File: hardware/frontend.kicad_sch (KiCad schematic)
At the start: 33 parts, among them J10 Conn_01x03_MountingPin, J11 Conn_01x11_MountingPin, J7 EXT_NTC, J8 EXT_NTC, J9 Conn_01x03_MountingPin, Q4 IPTC025N15NM6, Q5 IPTC025N15NM6, Q6 BSS127S, U5 BQ769x2

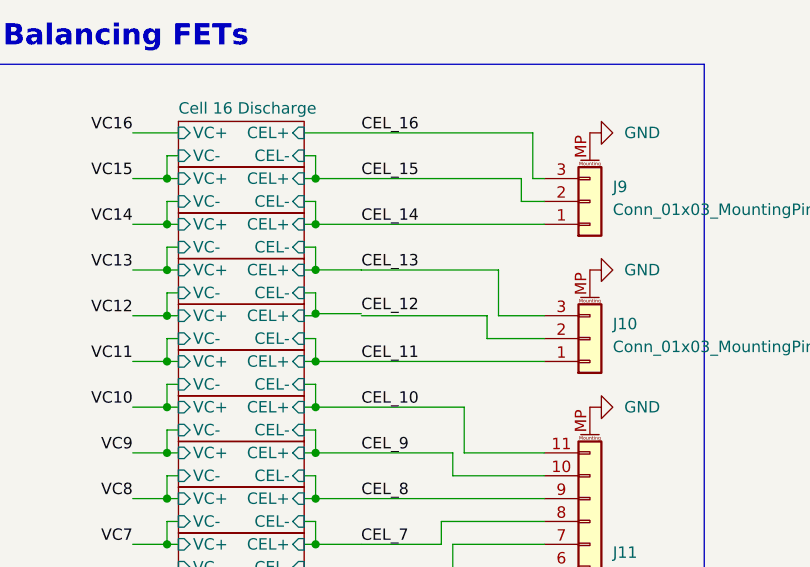
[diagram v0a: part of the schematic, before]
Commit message: Cell balancing sourcing and repositioning
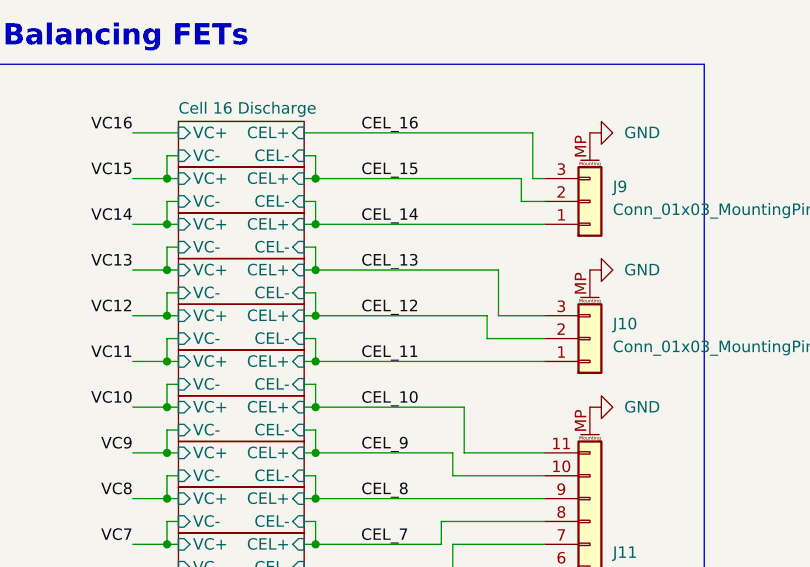
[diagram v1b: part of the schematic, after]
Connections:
- net CEL_12: now also J10.2 (Pin_2)
- net CEL_13: now also J10.3 (Pin_3)
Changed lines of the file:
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@@
+	)
+	(junction
+		(at 350.52 87.63)
+		(diameter 0)
+		(color 0 0 0 0)
 	)
 	(junction
@@
 	)
 	(junction
-		(at 350.52 87.6153)
-		(diameter 0)
-		(color 0 0 0 0)
-	)
-	(junction
 		(at 350.52 97.79)
 		(diameter 0)
@@
 	)
 	(junction
+		(at 350.52 92.71)
+		(diameter 0)
+		(color 0 0 0 0)
+	)
+	(junction
 		(at 334.01 107.95)
 		(diameter 0)
@@
 	)
 	(junction
-		(at 350.52 92.48)
-		(diameter 0)
-		(color 0 0 0 0)
-	)
-	(junction
 		(at 334.01 123.19)
 		(diameter 0)
@@
 	(wire
 		(pts
-			(xy 350.52 92.48) (xy 350.52 90.17)
-		)
-		(stroke
-			(width 0)
-			(type default)
-		)
-	)
-	(wire
-		(pts
 			(xy 349.25 72.39) (xy 374.65 72.39)
 		)
@@
 	(wire
 		(pts
-			(xy 355.6 92.71) (xy 369.57 92.71)
-		)
-		(stroke
-			(width 0)
-			(type default)
-		)
-	)
-	(wire
-		(pts
-			(xy 350.52 87.63) (xy 350.52 87.6153)
+			(xy 350.52 85.09) (xy 350.52 87.63)
 		)
 		(stroke
@@
 	(wire
 		(pts
-			(xy 350.52 87.6153) (xy 355.6 87.6153)
-		)
-		(stroke
-			(width 0)
-			(type default)
-		)
-	)
-	(wire
-		(pts
 			(xy 180.34 193.04) (xy 180.34 203.2)
 		)
@@
 	(wire
 		(pts
-			(xy 370.84 87.63) (xy 355.6 87.63)
-		)
-		(stroke
-			(width 0)
-			(type default)
-		)
-	)
-	(wire
-		(pts
 			(xy 334.01 157.48) (xy 334.01 160.02)
 		)
@@
 	(wire
 		(pts
+			(xy 350.52 87.63) (xy 370.84 87.63)
+		)
+		(stroke
+			(width 0)
+			(type default)
+		)
+	)
+	(wire
+		(pts
 			(xy 364.49 118.11) (xy 364.49 115.57)
 		)
@@
 	(wire
 		(pts
-			(xy 350.52 87.6153) (xy 350.52 85.09)
-		)
-		(stroke
-			(width 0)
-			(type default)
-		)
-	)
-	(wire
-		(pts
 			(xy 349.25 138.43) (xy 350.52 138.43)
 		)
@@
 	(wire
 		(pts
-			(xy 350.52 92.48) (xy 355.6 92.48)
+			(xy 350.52 92.71) (xy 369.57 92.71)
 		)
 		(stroke
@@
 	(wire
 		(pts
-			(xy 350.52 92.71) (xy 350.52 92.48)
+			(xy 350.52 90.17) (xy 350.52 92.71)
 		)
 		(stroke
@@
 	)
 	(label "CEL_13"
-		(at 355.6 87.6153 0)
+		(at 355.6 87.63 0)
 		(effects
 			(font
@@
 	)
 	(label "CEL_12"
-		(at 355.6 92.48 0)
-		(effects
-			(font
+		(at 355.6 92.71 0)
+		(effects
+			(font
